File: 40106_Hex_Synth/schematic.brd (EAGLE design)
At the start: 92.9 x 49 mm, 39 parts, among them J15 POWER_JACK, U1 CD40106BE

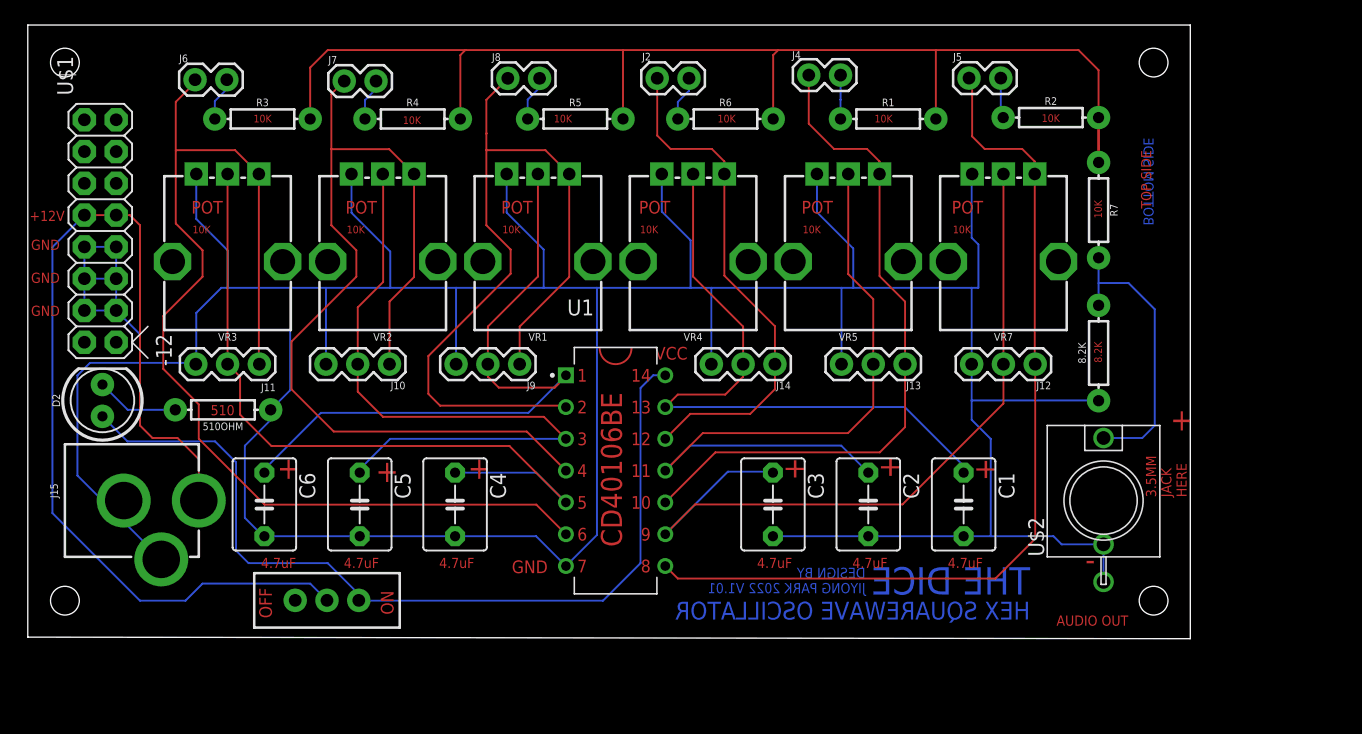
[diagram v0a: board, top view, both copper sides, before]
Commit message: Add files via upload
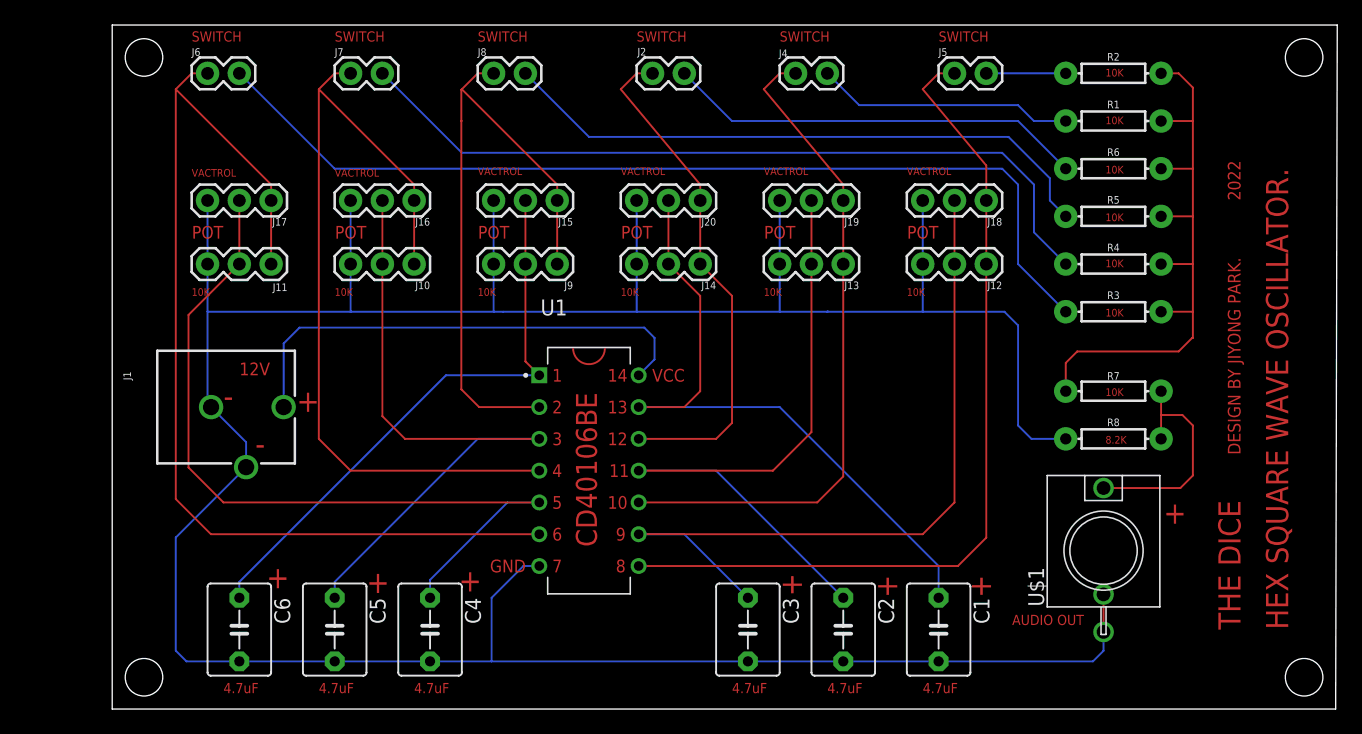
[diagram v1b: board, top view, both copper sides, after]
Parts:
- removed 510OHM, 8.2K: (no value), SparkFun-Resistors:AXIAL-0.3
- removed D2: (no value), SparkFun-LED:LED_5MM
- removed S1: (no value), SparkFun-Switches:SWITCH_SPDT_PTH_11.6X4.0MM
- removed U$2: WQP-PJ301M-12_JACK, thonkiconn:WQP-PJ301M-12_JACK
- removed VR1, VR2, VR3, VR4, VR5, VR7: 10k, SparkFun-Resistors:POT-PTH-ALPS
- added J1: POWER_JACKPTH_BREAD, SparkFun-Connectors:POWER_JACK_PTH_BREAD
- added J16, J17, J18, J19, J20: (no value), SparkFun-Connectors:1X03
- added R8: (no value), SparkFun-Resistors:AXIAL-0.3
- J15: value POWER_JACK -> (none); device SparkFun-Connectors:POWER_JACK_PTH -> SparkFun-Connectors:1X03
- U$1: value POWER_SIMPLE16 -> WQP-PJ301M-12_JACK; device eurorack:POWER_16 -> thonkiconn:WQP-PJ301M-12_JACK
- moved U$1 83.4 mm to (97.0, 66.0), turned to 0 degrees
- moved R3 69.7 mm to (97.8, 85.1)
- moved R4 57.2 mm to (97.8, 88.9)
- moved J15 48.7 mm to (53.3, 94.0), turned to 180 degrees
- moved R5 43.7 mm to (97.8, 92.7)
- moved R6 31.3 mm to (97.8, 96.5)
- moved R1 18.0 mm to (97.8, 100.3)
- moved R7 14.5 mm to (97.8, 78.7), turned to 180 degrees
- moved C1 10.2 mm to (83.8, 59.7)
- moved C2 10.2 mm to (76.2, 59.7)
- moved C3 10.2 mm to (68.6, 59.7)
- moved C4 10.2 mm to (43.2, 59.7)
- moved C5 10.2 mm to (35.6, 59.7)
- moved C6 10.2 mm to (27.9, 59.7)
- moved J14 9.98 mm to (64.8, 88.9)
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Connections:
- removed net N$1 (its old number): 510OHM.P$2, D2.K
- removed net N$24: J15.PWR, S1.2, U$1.10, U$1.9
- removed net N$25: D2.A, S1.3, U1.14
- new net VCC: J1.PWR, U1.14
- net GND: now also J1.GND, J1.GNDBREAK, J15.3, J16.3, J17.3, J18.3, J19.3, J20.3, R8.P$1, U$1.P$2, U$1.P$3; no longer 510OHM.P$1, 8.2K.P$1, J15.GND, J15.GNDBREAK, U$1.3, U$1.4, U$1.5, U$1.6, U$1.7, U$1.8, U$2.P$2, U$2.P$3, VR1.P$3, VR2.P$3, VR3.P$3, VR4.P$3, VR5.P$3, VR7.P$3
- net N$15: now also J19.1; no longer VR5.P$1
- net N$16: now also J18.2; no longer VR7.P$2
- net N$17: now also J17.1; no longer VR3.P$1
- net N$18: now also J16.1; no longer VR2.P$1
- net N$19: now also J15.1; no longer VR1.P$1
- net N$2: now also J20.2; no longer VR4.P$2
- net N$21: now also R8.P$2, U$1.P$1; no longer 8.2K.P$2, U$2.P$1
- net N$3: now also J20.1; no longer VR4.P$1
- net N$5: now also J18.1; no longer VR7.P$1
- net N$6: now also J17.2; no longer VR3.P$2
- net N$7: now also J16.2; no longer VR2.P$2
- net N$8: now also J15.2; no longer VR1.P$2
- net N$9: now also J19.2; no longer VR5.P$2
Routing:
- net GND: track 334.5 -> 250.9 mm
- net N$24: track 80.7 -> 0.00 mm
- net N$13: track 3.53 -> 77.7 mm
- net N$25: track 71.2 -> 0.00 mm
- net N$12: track 3.39 -> 63.2 mm
- net N$1: track 101.7 -> 49.0 mm
- net N$11: track 3.64 -> 49.0 mm
- net VCC: track 0.00 -> 39.1 mm
- net N$14: track 3.62 -> 33.6 mm
- net N$4: track 3.51 -> 20.6 mm
- net N$19: track 65.2 -> 51.0 mm
- net N$18: track 76.1 -> 66.8 mm
- net N$1 (its old number): track 6.66 -> 0.00 mm
- net N$6: track 58.4 -> 64.9 mm
- net N$8: track 52.7 -> 46.5 mm
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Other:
- board size 92.9 x 49 mm -> 97.9 x 54.7 mm
- board text added: "12V"
- board text added: "2022"
- board text added: "DESIGN BY JIYONG PARK."
- board text added: "HEX SQUARE WAVE OSCILLATOR."
- board text added: "SWITCH"
- board text added: "VACTROL"
- board text removed: "+12V"
- board text removed: "3.5MM JACK HERE"
- board text removed: "510"
- board text removed: "BOTTOM SIDE"
- board text removed: "DESIGN BY JIYONG PARK 2022 V1.01"
- board text removed: "HEX SQUAREWAVE OSCILLATOR"
- board text removed: "OFF"
- board text removed: "ON"
- board text removed: "TOP SIDE"

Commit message: Add files via upload
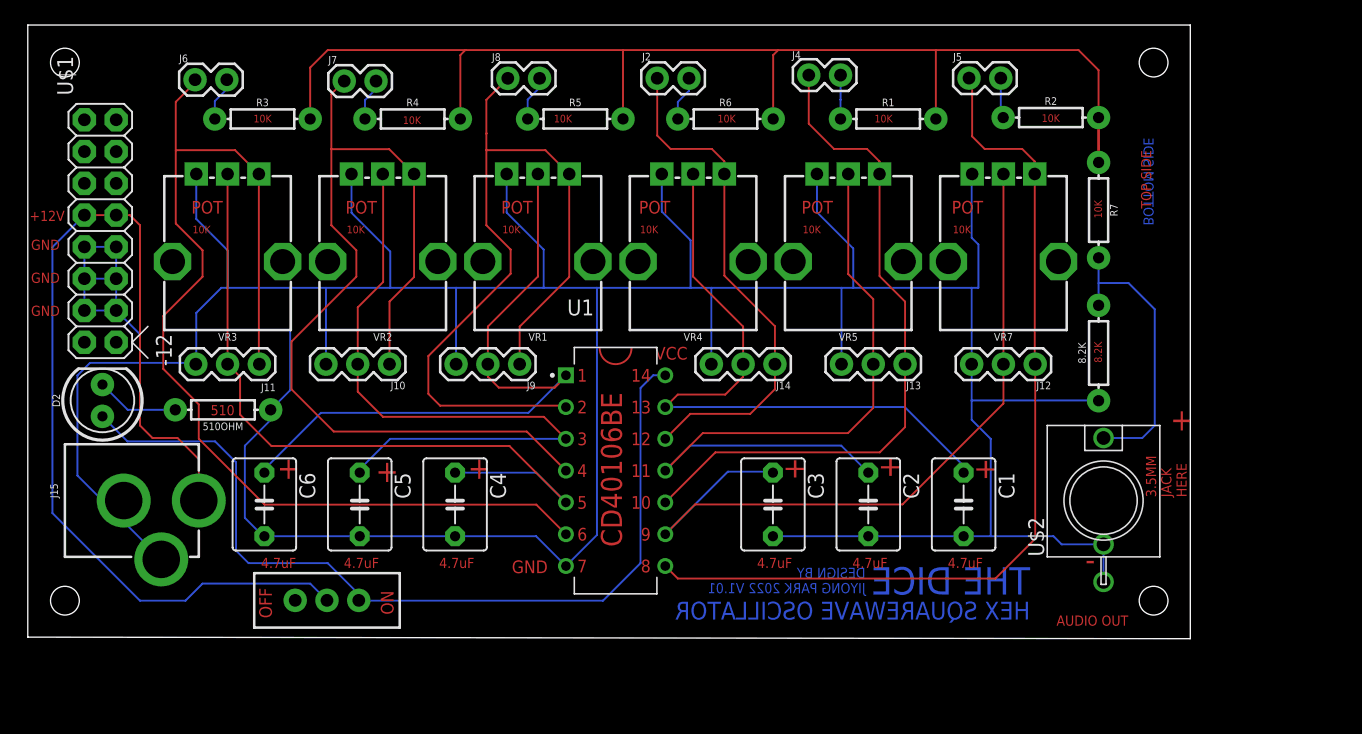
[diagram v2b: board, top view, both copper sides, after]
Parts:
- removed J1: POWER_JACKPTH_BREAD, SparkFun-Connectors:POWER_JACK_PTH_BREAD
- removed J16, J17, J18, J19, J20: (no value), SparkFun-Connectors:1X03
- removed R8: (no value), SparkFun-Resistors:AXIAL-0.3
- added 510OHM, 8.2K: (no value), SparkFun-Resistors:AXIAL-0.3
- added D2: (no value), SparkFun-LED:LED_5MM
- added S1: (no value), SparkFun-Switches:SWITCH_SPDT_PTH_11.6X4.0MM
- added U$2: WQP-PJ301M-12_JACK, thonkiconn:WQP-PJ301M-12_JACK
- added VR1, VR2, VR3, VR4, VR5, VR7: 10k, SparkFun-Resistors:POT-PTH-ALPS
- J15: value (none) -> POWER_JACK; device SparkFun-Connectors:1X03 -> SparkFun-Connectors:POWER_JACK_PTH
- U$1: value WQP-PJ301M-12_JACK -> POWER_SIMPLE16; device thonkiconn:WQP-PJ301M-12_JACK -> eurorack:POWER_16
- moved U$1 83.4 mm to (16.8, 89.0), turned to 90 degrees
- moved R3 69.7 mm to (29.8, 100.5)
- moved R4 57.2 mm to (41.8, 100.5)
- moved J15 48.7 mm to (11.0, 70.0), turned to 270 degrees
- moved R5 43.7 mm to (54.8, 100.5)
- moved R6 31.3 mm to (66.8, 100.5)
- moved R1 18.0 mm to (79.8, 100.5)
- moved R7 14.5 mm to (96.6, 93.2), turned to 90 degrees
- moved C1 10.2 mm to (85.8, 69.7)
- moved C2 10.2 mm to (78.2, 69.7)
- moved C3 10.2 mm to (70.6, 69.7)
- moved C4 10.2 mm to (45.2, 69.7)
- moved C5 10.2 mm to (37.6, 69.7)
- moved C6 10.2 mm to (29.9, 69.7)
- moved J14 9.98 mm to (70.7, 80.9)
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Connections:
- removed net VCC: J1.PWR, U1.14
- new net N$1: 510OHM.P$2, D2.K
- new net N$24: J15.PWR, S1.2, U$1.10, U$1.9
- new net N$25: D2.A, S1.3, U1.14
- net GND: now also 510OHM.P$1, 8.2K.P$1, J15.GND, J15.GNDBREAK, U$1.3, U$1.4, U$1.5, U$1.6, U$1.7, U$1.8, U$2.P$2, U$2.P$3, VR1.P$3, VR2.P$3, VR3.P$3, VR4.P$3, VR5.P$3, VR7.P$3; no longer J1.GND, J1.GNDBREAK, J15.3, J16.3, J17.3, J18.3, J19.3, J20.3, R8.P$1, U$1.P$2, U$1.P$3
- net N$15: now also VR5.P$1; no longer J19.1
- net N$16: now also VR7.P$2; no longer J18.2
- net N$17: now also VR3.P$1; no longer J17.1
- net N$18: now also VR2.P$1; no longer J16.1
- net N$19: now also VR1.P$1; no longer J15.1
- net N$2: now also VR4.P$2; no longer J20.2
- net N$21: now also 8.2K.P$2, U$2.P$1; no longer R8.P$2, U$1.P$1
- net N$3: now also VR4.P$1; no longer J20.1
- net N$5: now also VR7.P$1; no longer J18.1
- net N$6: now also VR3.P$2; no longer J17.2
- net N$7: now also VR2.P$2; no longer J16.2
- net N$8: now also VR1.P$2; no longer J15.2
- net N$9: now also VR5.P$2; no longer J19.2
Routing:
- net GND: track 250.9 -> 334.5 mm
- net N$24: track 0.00 -> 80.7 mm
- net N$13: track 77.7 -> 3.53 mm
- net N$25: track 0.00 -> 71.2 mm
- net N$12: track 63.2 -> 3.39 mm
- net N$23: track 49.0 -> 101.7 mm
- net N$11: track 49.0 -> 3.64 mm
- net VCC: track 39.1 -> 0.00 mm
- net N$14: track 33.6 -> 3.62 mm
- net N$4: track 20.6 -> 3.51 mm
- net N$19: track 51.0 -> 65.2 mm
- net N$18: track 66.8 -> 76.1 mm
- net N$1: track 0.00 -> 6.66 mm
- net N$6: track 64.9 -> 58.4 mm
- net N$8: track 46.5 -> 52.7 mm
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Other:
- board size 97.9 x 54.7 mm -> 92.9 x 49 mm
- board text added: "+12V"
- board text added: "3.5MM JACK HERE"
- board text added: "510"
- board text added: "BOTTOM SIDE"
- board text added: "DESIGN BY JIYONG PARK 2022 V1.01"
- board text added: "HEX SQUAREWAVE OSCILLATOR"
- board text added: "OFF"
- board text added: "ON"
- board text added: "TOP SIDE"
- board text removed: "12V"
- board text removed: "2022"
- board text removed: "DESIGN BY JIYONG PARK."
- board text removed: "HEX SQUARE WAVE OSCILLATOR."
- board text removed: "SWITCH"
- board text removed: "VACTROL"
